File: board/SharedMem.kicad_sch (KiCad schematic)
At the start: 10 parts, among them U19 HM628512LP-5, U20 HM628512LP-5, U21 HM628512LP-5, U22 HM628512LP-5, U23 74F139

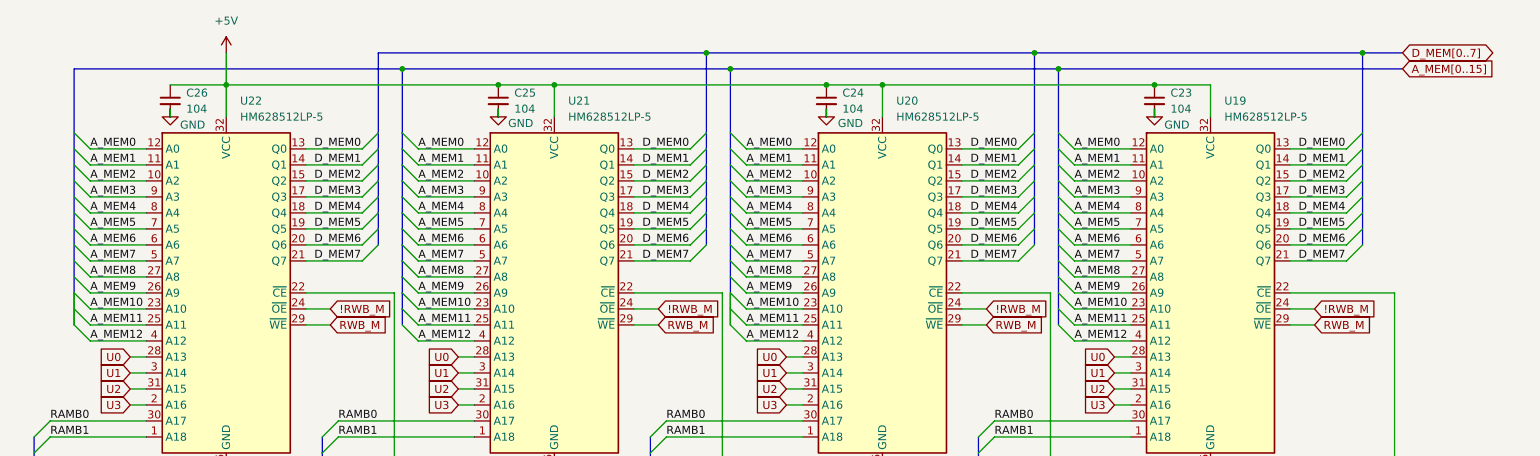
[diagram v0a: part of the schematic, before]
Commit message: V1.4E
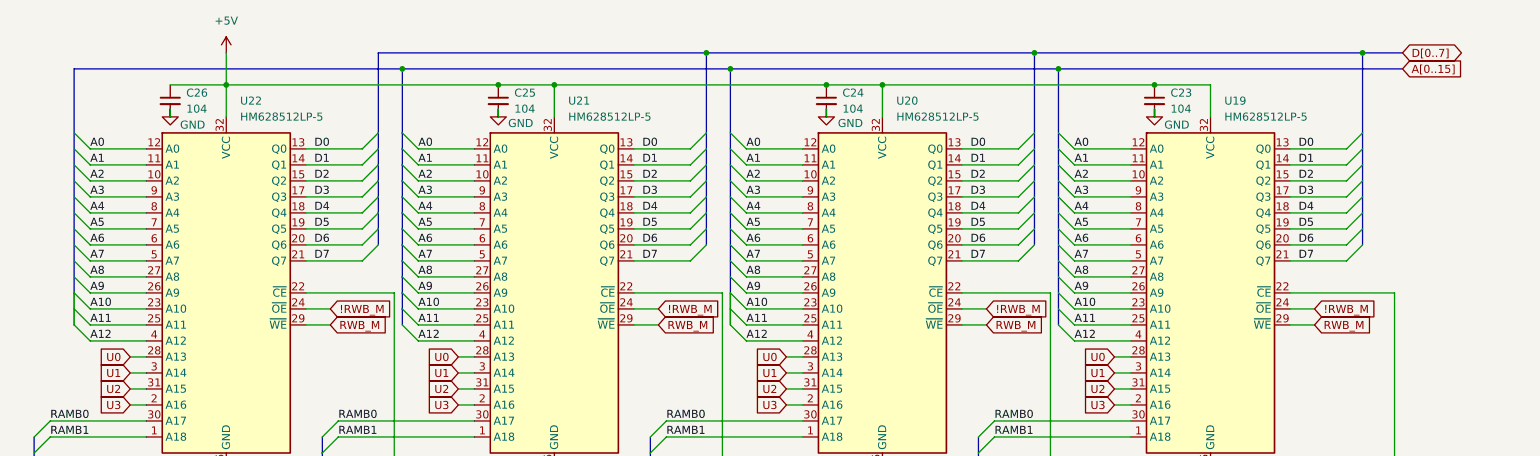
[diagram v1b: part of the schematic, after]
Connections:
- net A_MEM0 renamed A0
- net A_MEM1 renamed A1
- net A_MEM10 renamed A10
- net A_MEM11 renamed A11
- net A_MEM12 renamed A12
- net A_MEM2 renamed A2
- net A_MEM3 renamed A3
- net A_MEM4 renamed A4
- net A_MEM5 renamed A5
- net A_MEM6 renamed A6
- net A_MEM7 renamed A7
- net A_MEM8 renamed A8
- net A_MEM9 renamed A9
- net D_MEM0 renamed D0
- net D_MEM1 renamed D1
- net D_MEM2 renamed D2
- net D_MEM3 renamed D3
- net D_MEM4 renamed D4
- net D_MEM5 renamed D5
- net D_MEM6 renamed D6
- net D_MEM7 renamed D7
